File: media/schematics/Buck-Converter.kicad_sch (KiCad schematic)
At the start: 15 parts

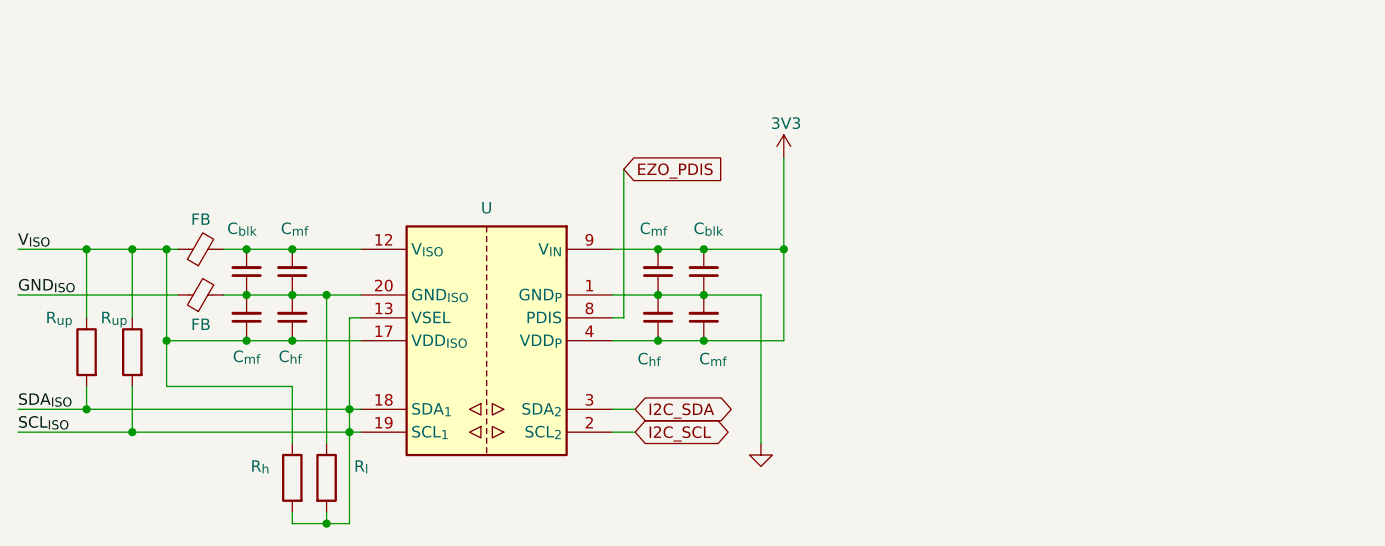
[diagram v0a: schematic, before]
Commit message: update
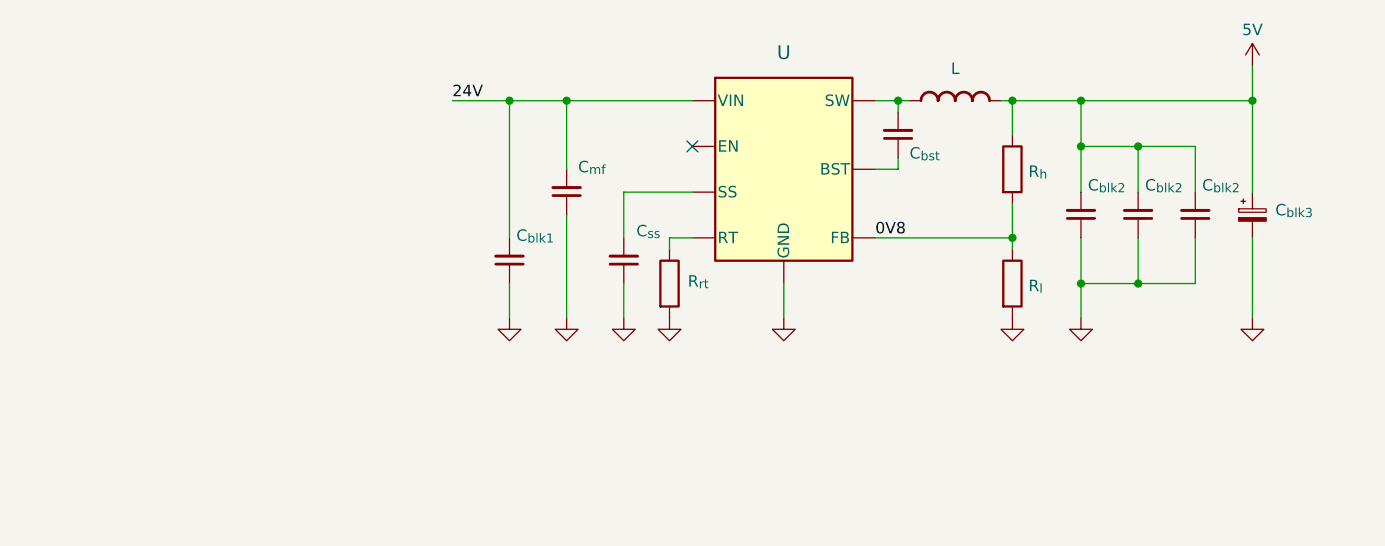
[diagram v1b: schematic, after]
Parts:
- removed C_{blk} (x2): 10μF, Coert-Vonk:CAP X5R 10μF ±10 16V 0805 Murata GRM, symbol Coert-Vonk:CAP X5R 10μF ±10% 16V 0805 Murata GRM
- removed C_{hf} (x2): 10nF, Coert-Vonk:CAP X7R 10nF ±10 16V 0402 Murata, symbol Coert-Vonk:CAP X7R 10nF ±10% 16V 0402 Murata
- removed C_{mf} (x4): 100nF, Coert-Vonk:CAP X7R 100nF ±10 50V 0402 Murata, symbol Coert-Vonk:CAP X7R 100nF ±10% 50V 0402 Murata
- removed FB (x2): 60Ω at 100MHz, symbol Coert-Vonk:FERRITE BEAD 20mΩ 60Ω 0603 TDK
- removed R_{h}: 16k9, Coert-Vonk:RES 0805 YAGEO, symbol Coert-Vonk:RES 16.9kΩ ±1% 1/8W 0805 Yageo
- removed R_{up} (x2): 2k2, Coert-Vonk:RES 0805 YAGEO, symbol Coert-Vonk:RES 2.2kΩ ±1% 1/8W 0805 Yageo
- removed U: ADM3260, Coert-Vonk:IC ISOLTR 2.5KV 2CH I2C 20SSOP ADM3260, symbol Coert-Vonk:IC ISOLTR 2.5KV 2CH I2C 20SSOP ADM3260
- added C_{blk1}: 10μF, Coert-Vonk:CAP X7R 10μF ±10 50V 1206 Murata GRT, symbol Coert-Vonk:CAP X7R 10μF ±10% 50V 1206 Murata GRT
- added C_{blk2} (x3): 10μF, Coert-Vonk:CAP X5R 10μF ±10 16V 0805 Murata GRM, symbol Coert-Vonk:CAP X5R 10μF ±10% 16V 0805 Murata GRM
- added C_{blk3}: 220μF, Coert-Vonk:CAP ALUM-POLY 220μF ±20 16V Panasonic, symbol Coert-Vonk:CAP ALUM-POLY 220μF ±20% 16V Panasonic
- added C_{bst}, C_{mf}: 100nF, Coert-Vonk:CAP X7R 100nF ±10 50V 0402 Murata, symbol Coert-Vonk:CAP X7R 100nF ±10% 50V 0402 Murata
- added C_{ss}: 33nF, Coert-Vonk:CAP X7R 33nF ±10 50V 0805 Kemet, symbol Coert-Vonk:CAP X7R 33nF ±10% 50V 0805 Kemet
- added L: 10µH, Coert-Vonk:IND 10µH 5.6A 21mΩ, symbol Coert-Vonk:IND 10µH 5.6A 21mΩ
- added R_{h}: 52k3, Coert-Vonk:RES 0805 YAGEO, symbol Coert-Vonk:RES 52.3kΩ ±1% 1/8W 0805 Yageo
- added R_{rt}: 21k, Coert-Vonk:RES 0805 YAGEO, symbol Coert-Vonk:RES 21kΩ ±1% 1/8W 0805 Yageo
- added U: TPS62933, Coert-Vonk:REG ADJ 3A BUCK TPS62933 SOT583, symbol Coert-Vonk:REG ADJ 3A BUCK TPS62933 SOT583
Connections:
- net SCL_{ISO} is gone; now on net GND: R_{l}.1
- net GND: now also C_{blk1}.1, C_{blk2}.1, C_{blk2}.1, C_{blk2}.1, C_{blk3}.2, C_{mf}.1, C_{ss}.1, R_{rt}.1, U.4 (GND)
- net 0V8: now reaches R_{l}.2
- net 0V8: now also R_{h}.1, U.8 (FB)
- new net: C_{bst}.2, L.1, U.5 (SW)
- new net: C_{bst}.1, U.6 (BST)
- new net: C_{ss}.2, U.7 (SS)
- new net: R_{rt}.2, U.1 (RT)
- new net 24V: C_{blk1}.2, C_{mf}.2, U.3 (VIN)
- new net 5V: C_{blk2}.2, C_{blk2}.2, C_{blk2}.2, C_{blk3}.1, L.2, R_{h}.2
- no-connect marks 0 -> 1
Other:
- title: OPNhydro ADM3260 -> OPNhydro
